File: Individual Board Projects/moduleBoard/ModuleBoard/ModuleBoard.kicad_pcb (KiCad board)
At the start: 2 copper layers, 74 x 85.4 mm, 18 parts, among them IC1 MSPM0C1103SDGS20R, J1 Rotation Servo, J2 Extention Servo, J3 Debug, J4 5x2.54mm+2xBus, J5 5x2.54mm+2xBus, J6 5x2.54mm+2xBus, J7 5x2.54mm+2xBus, J8 5x2.54mm+2xBus, J9 5x2.54mm+2xBus, U1 FZ2812-5050

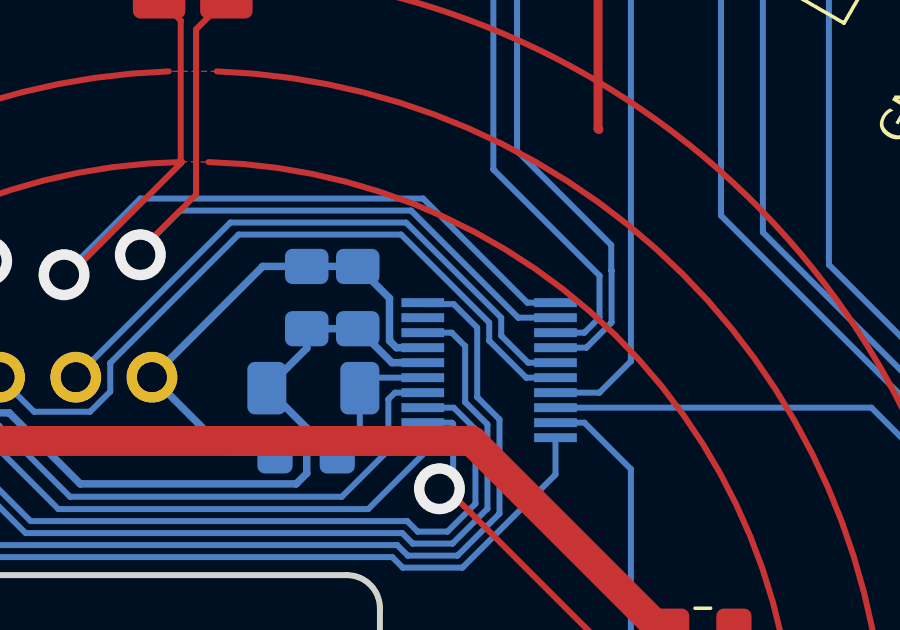
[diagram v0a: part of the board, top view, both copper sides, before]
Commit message: Interconnect Board
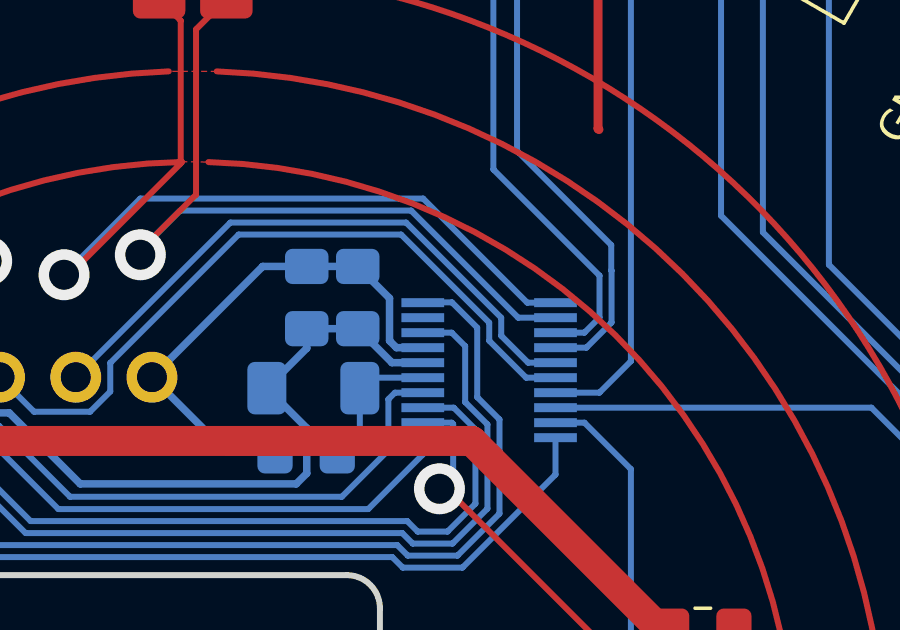
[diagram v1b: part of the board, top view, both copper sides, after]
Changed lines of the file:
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@@
 	)
 	(segment
-		(start 198.6125 76.571529)
-		(end 199.354528 77.313559)
+		(start 197.77 73.41)
+		(end 198.6125 74.2525)
 		(width 0.2)
 		(layer "B.Cu")
@@
 	)
 	(segment
-		(start 196.847 73.469)
-		(end 197.829 73.469)
+		(start 199.354528 77.313559)
+		(end 199.354528 80.452371)
+		(width 0.2)
+		(layer "B.Cu")
+		(net 13)
+	)
+	(segment
+		(start 197.955009 81.85189)
+		(end 196.297324 81.85189)
+		(width 0.2)
+		(layer "B.Cu")
+		(net 13)
+	)
+	(segment
+		(start 195.946393 81.50096)
+		(end 182.33096 81.50096)
+		(width 0.2)
+		(layer "B.Cu")
+		(net 13)
+	)
+	(segment
+		(start 196.808 73.41)
+		(end 197.77 73.41)
+		(width 0.2)
+		(layer "B.Cu")
+		(net 13)
+	)
+	(segment
+		(start 182.33096 81.50096)
+		(end 180.75 79.92)
 		(width 0.2)
 		(layer "B.Cu")
@@
 	)
 	(segment
+		(start 198.6125 74.2525)
+		(end 198.6125 76.571529)
+		(width 0.2)
+		(layer "B.Cu")
+		(net 13)
+	)
+	(segment
+		(start 198.6125 76.571529)
+		(end 199.354528 77.313559)
+		(width 0.2)
+		(layer "B.Cu")
+		(net 13)
+	)
+	(segment
 		(start 199.354528 80.452371)
 		(end 197.955009 81.85189)
@@
 	)
 	(segment
-		(start 197.829 73.469)
-		(end 198.6125 74.2525)
+		(start 196.798 73.42)
+		(end 196.808 73.41)
 		(width 0.2)
 		(layer "B.Cu")
-		(net 13)
-	)
-	(segment
-		(start 198.6125 74.2525)
-		(end 198.6125 76.571529)
-		(width 0.2)
-		(layer "B.Cu")
-		(net 13)
-	)
-	(segment
-		(start 195.946393 81.50096)
-		(end 182.33096 81.50096)
-		(width 0.2)
-		(layer "B.Cu")
-		(net 13)
-	)
-	(segment
-		(start 197.955009 81.85189)
-		(end 196.297324 81.85189)
-		(width 0.2)
-		(layer "B.Cu")
-		(net 13)
-	)
-	(segment
-		(start 199.354528 77.313559)
-		(end 199.354528 80.452371)
-		(width 0.2)
-		(layer "B.Cu")
-		(net 13)
-	)
-	(segment
-		(start 182.33096 81.50096)
-		(end 180.75 79.92)
-		(width 0.2)
-		(layer "B.Cu")
